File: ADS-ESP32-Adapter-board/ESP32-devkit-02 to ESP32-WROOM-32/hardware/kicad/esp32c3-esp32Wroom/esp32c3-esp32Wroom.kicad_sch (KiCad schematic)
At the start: 4 parts, among them J1 Conn_01x15_esp32_devkit_V1_el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, J2 Conn_01x15_esp32_devkit_V1_el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, J3 Conn_01x15_esp32_c3_devkit_02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, J4 Conn_01x15_esp32_c3_devkit_02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

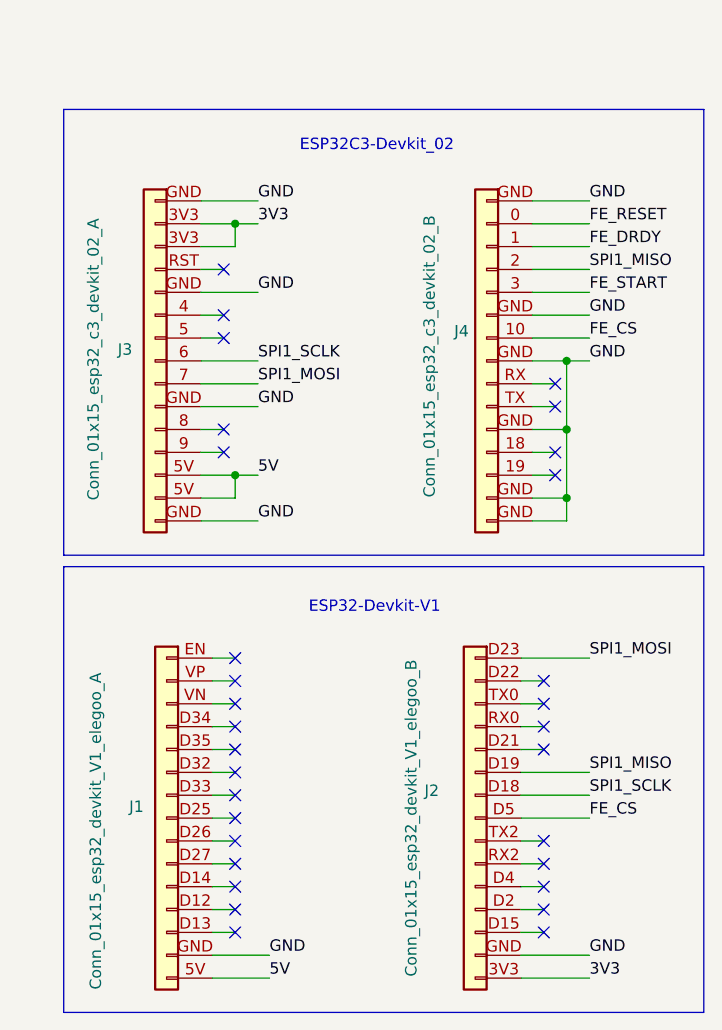
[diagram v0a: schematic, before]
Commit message: modified
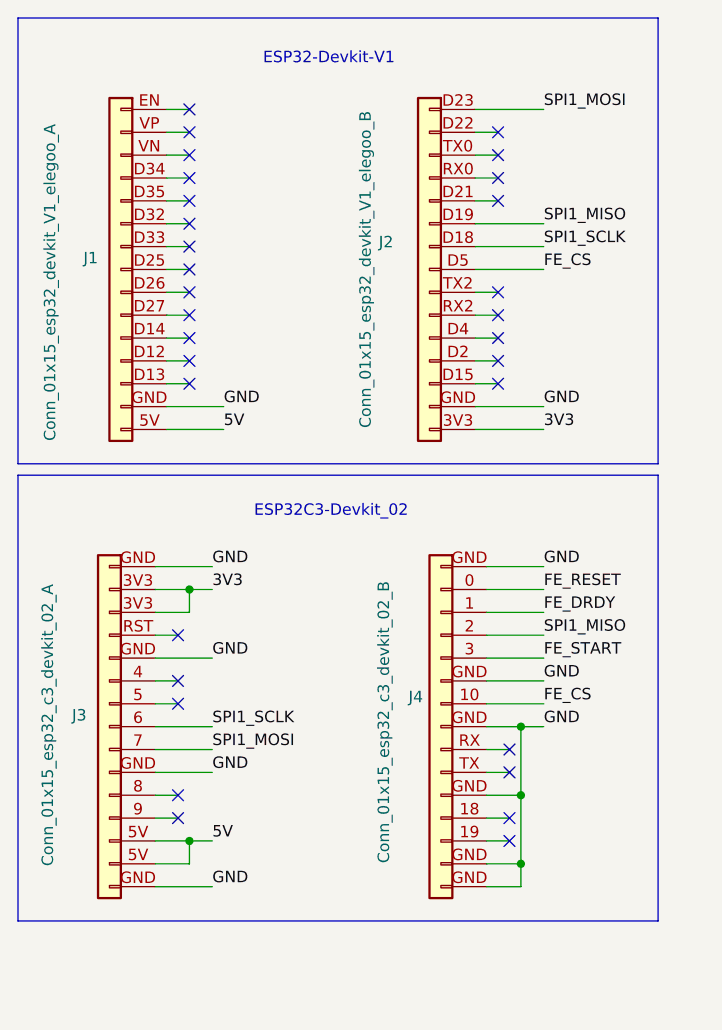
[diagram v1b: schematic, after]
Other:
- company: (none) -> BIOMEC UMA dpto Hardware
- title: (none) -> ESP32-C3-DevkitC-02
- moved on the sheet: J1, J2, J3, J4
